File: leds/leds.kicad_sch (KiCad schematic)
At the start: 0 parts

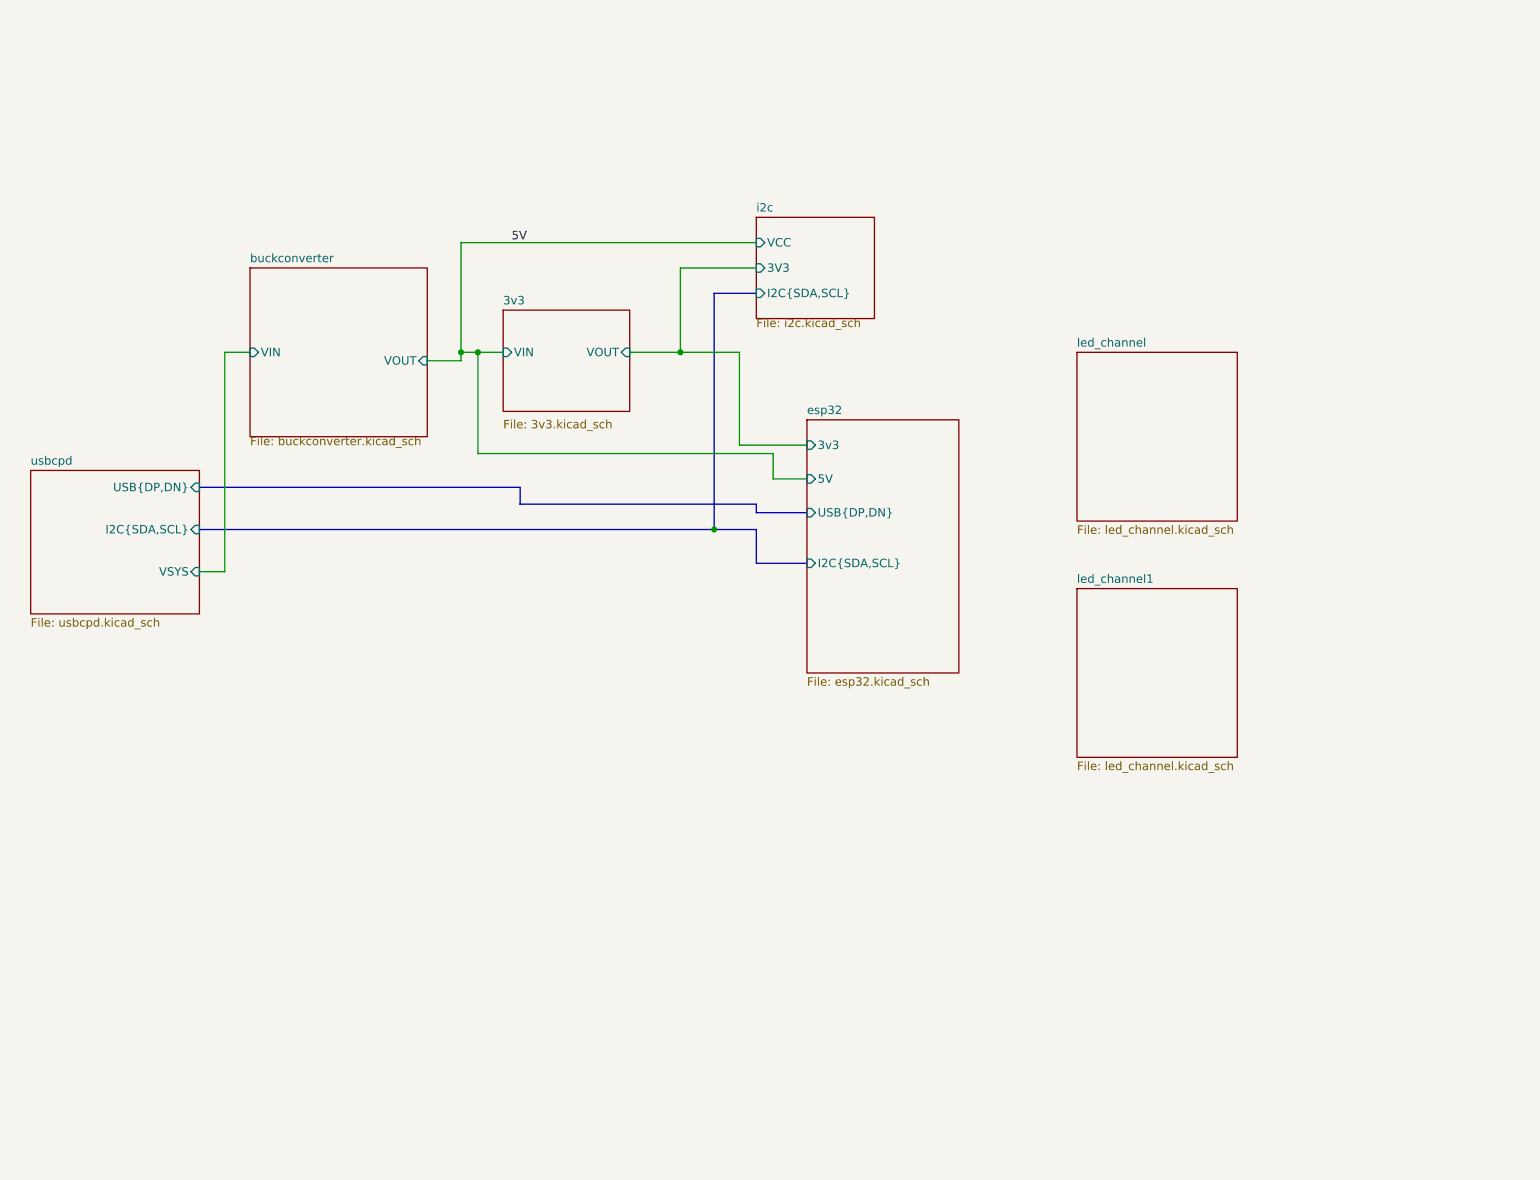
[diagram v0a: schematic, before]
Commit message: first draft
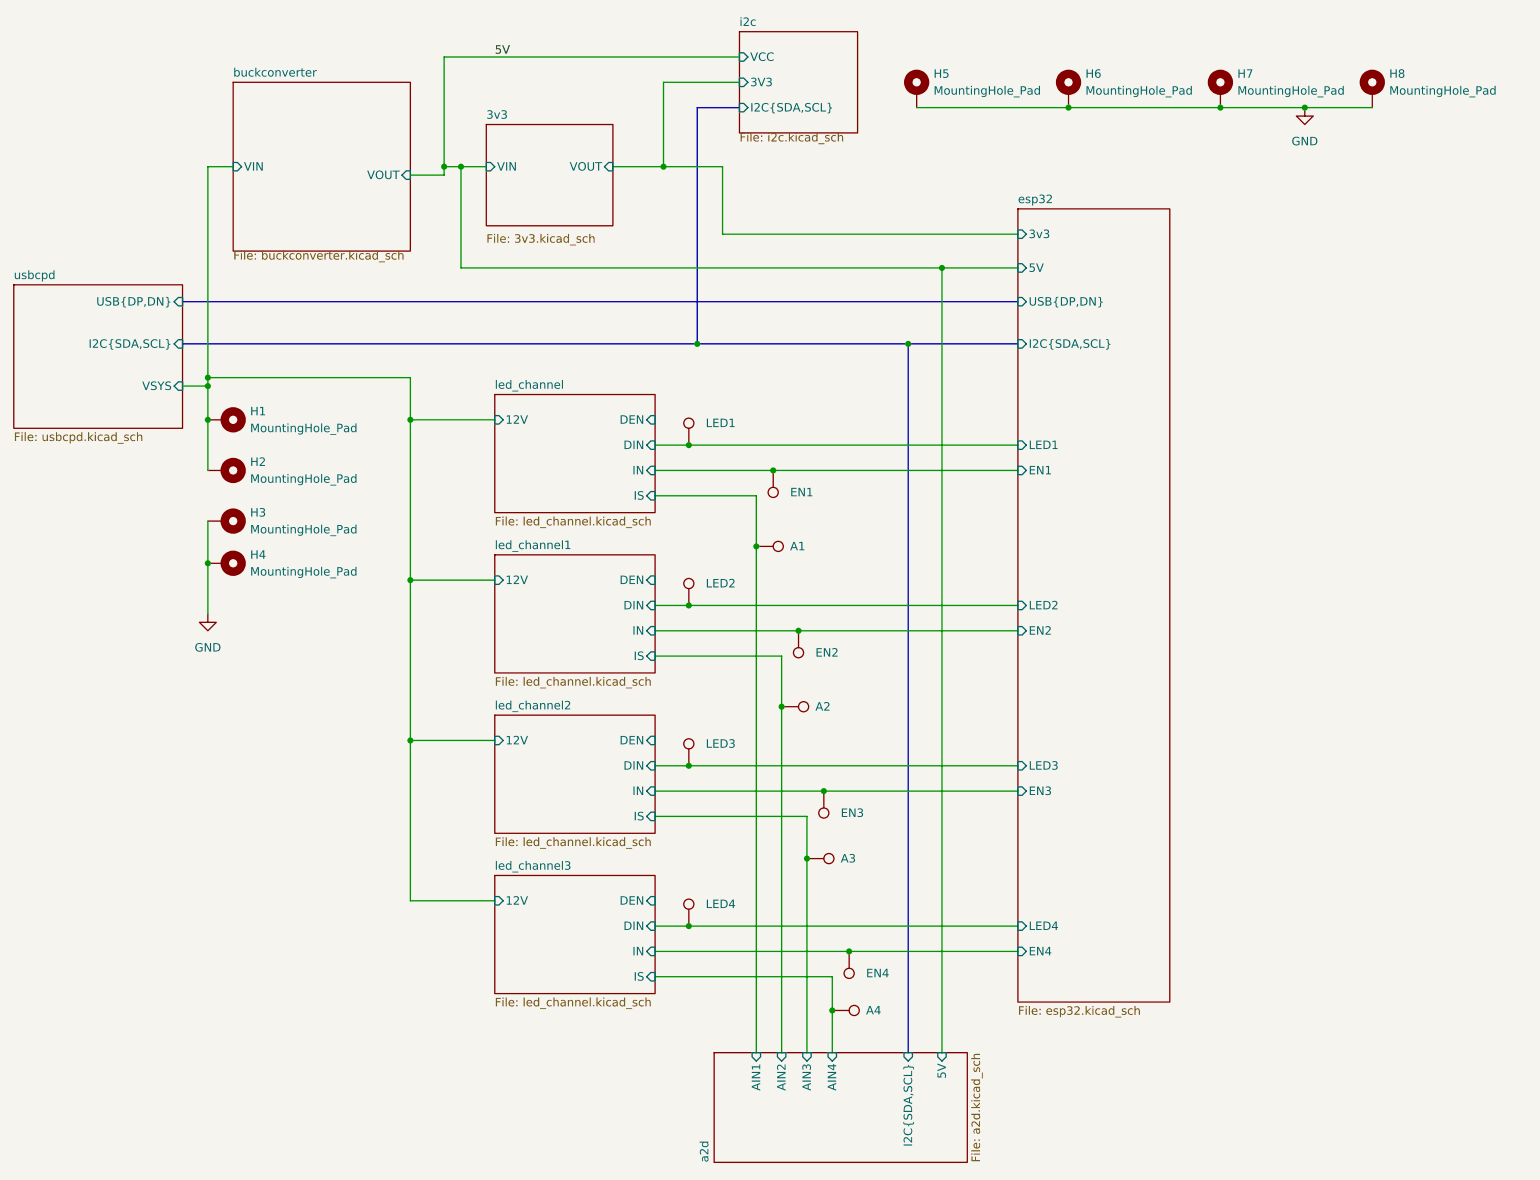
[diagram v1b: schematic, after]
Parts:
- added H1, H2, H3, H4: MountingHole_Pad, MountingHole:MountingHole_4mm_Pad_Via, symbol Mechanical:MountingHole_Pad
- added H5, H6, H7, H8: MountingHole_Pad, MountingHole:MountingHole_3.2mm_M3_Pad_Via, symbol Mechanical:MountingHole_Pad
- added TP10, TP11, TP12, TP13, TP14, TP15, TP16, TP5, TP6, TP7, TP8, TP9: LabeledTestPoint, easyeda2kicad:LabeledTestPoint, symbol easyeda2kicad:LabeledTestPoint
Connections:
- net buckconverter/VIN: now also H1.1, H2.1
- new net GND: H3.1, H4.1, H5.1, H6.1, H7.1, H8.1
- new net a2d/AIN1: TP13.1
- new net a2d/AIN2: TP14.1
- new net a2d/AIN3: TP15.1
- new net a2d/AIN4: TP16.1
- new net esp32/EN1: TP9.1
- new net esp32/EN2: TP10.1
- new net esp32/EN3: TP11.1
- new net esp32/EN4: TP12.1
- new net esp32/LED1: TP5.1
- new net esp32/LED2: TP6.1
- new net esp32/LED3: TP7.1
- new net esp32/LED4: TP8.1
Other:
- added sheet a2d (a2d.kicad_sch)
- added sheet led_channel2 (led_channel.kicad_sch)
- added sheet led_channel3 (led_channel.kicad_sch)
- sheet esp32 ports: added EN1, EN2, EN3, EN4, LED1, LED2, LED3, LED4; removed none
- sheet led_channel ports: added 12V, DEN, DIN, IN, IS; removed none
- sheet led_channel1 ports: added 12V, DEN, DIN, IN, IS; removed none
